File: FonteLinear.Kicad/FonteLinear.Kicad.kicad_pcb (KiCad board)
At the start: 2 copper layers, 26 parts, among them J1 Conn_01x03_Male, J2 Conn_01x02_Male, J3 Conn_01x02_Male, J4 Conn_01x02_Male, J5 Conn_01x02_Male, U1 LM317_TO39, U2 LM7805_TO220, U3 LM7815_TO220, U4 LM7915_TO220

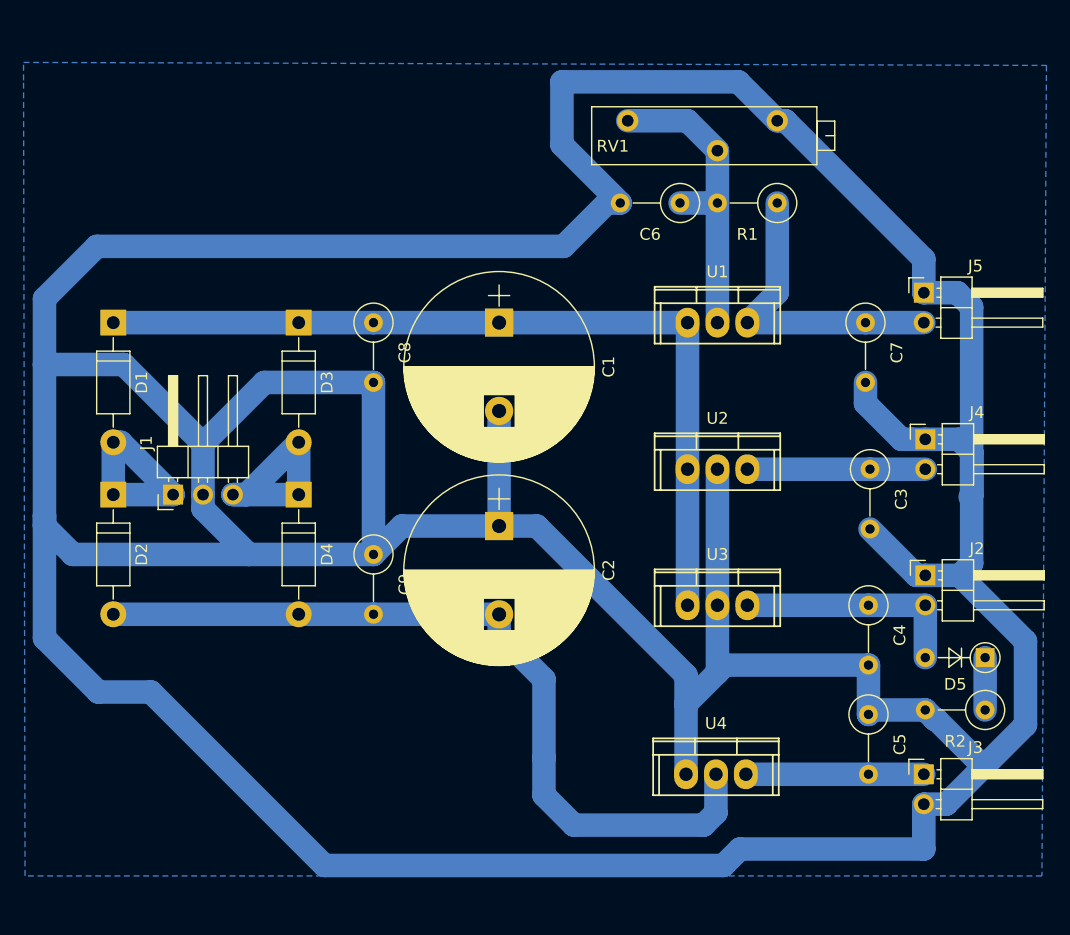
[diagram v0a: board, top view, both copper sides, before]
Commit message: Add files via upload
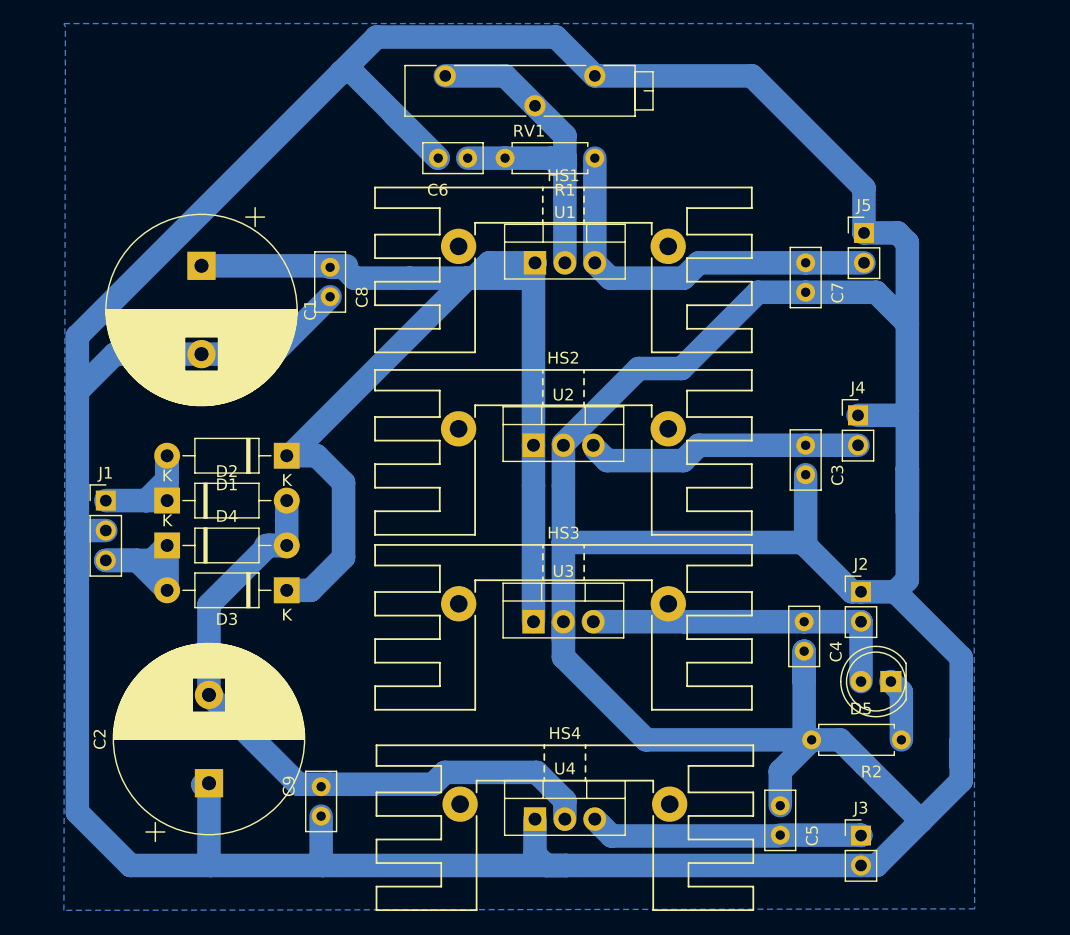
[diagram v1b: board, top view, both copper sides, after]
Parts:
- added HS1: Heatsink, Heatsinks:Heatsink_Stonecold_HS-132_32x14mm_2xFixation1.5mm, F.Cu at (236.6, 106.7)
- added HS2: Heatsink, Heatsinks:Heatsink_Stonecold_HS-132_32x14mm_2xFixation1.5mm, F.Cu at (236.6, 122.2)
- added HS3: Heatsink, Heatsinks:Heatsink_Stonecold_HS-132_32x14mm_2xFixation1.5mm, F.Cu at (236.6, 137.0)
- added HS4: Heatsink, Heatsinks:Heatsink_Stonecold_HS-132_32x14mm_2xFixation1.5mm, F.Cu at (236.7, 154.1)
- C1, C2: footprint Capacitors_THT:CP_Radial_D16.0mm_P7.50mm -> Capacitor_THT:CP_Radial_D16.0mm_P7.50mm
- C3, C4, C5, C6, C7, C8, C9: footprint Resistors_THT:R_Axial_DIN0309_L9.0mm_D3.2mm_P5.08mm_Vertical -> Capacitors_THT:C_Disc_D5.0mm_W2.5mm_P2.50mm
- D1, D2, D3, D4: footprint Diodes_THT:D_DO-41_SOD81_P10.16mm_Horizontal -> Diode_THT:D_DO-41_SOD81_P10.16mm_Horizontal
- D5: footprint Diodes_THT:D_DO-35_SOD27_P5.08mm_Vertical_AnodeUp -> LEDs:LED_D5.0mm
- J1: footprint Pin_Headers:Pin_Header_Angled_1x03_Pitch2.54mm -> Connector_PinHeader_2.54mm:PinHeader_1x03_P2.54mm_Vertical
- J2, J3, J4, J5: footprint Pin_Headers:Pin_Header_Angled_1x02_Pitch2.54mm -> Connector_PinHeader_2.54mm:PinHeader_1x02_P2.54mm_Vertical
- R1, R2: footprint Resistors_THT:R_Axial_DIN0309_L9.0mm_D3.2mm_P5.08mm_Vertical -> Resistors_THT:R_Axial_DIN0207_L6.3mm_D2.5mm_P7.62mm_Horizontal
- RV1: footprint Potentiometers:Potentiometer_Trimmer_Vishay_43 -> Potentiometer_THT:Potentiometer_Bourns_3005_Horizontal
- U1, U2, U3, U4: footprint Power_Integrations:TO-220 -> Package_TO_SOT_THT:TO-220-3_Vertical
- moved C2 32.9 mm to (206.5, 152.3), turned to 90 degrees
- moved C1 25.7 mm to (205.9, 108.3)
- moved D3 22.8 mm to (213.1, 135.9), turned to 180 degrees
- moved C9 22.7 mm to (216.0, 155.1), turned to 90 degrees
- moved D1 18.6 mm to (213.1, 124.5), turned to 180 degrees
- moved C6 18.4 mm to (228.5, 99.2)
- moved U1 16.3 mm to (234.2, 108.1)
- moved R1 16.0 mm to (239.3, 99.2)
- moved RV1 16.0 mm to (226.6, 92.2)
- moved U4 15.8 mm to (234.2, 155.3)
- moved U2 15.8 mm to (234.1, 123.6)
- moved U3 15.7 mm to (234.1, 138.6)
- moved D4 12.0 mm to (202.9, 132.1), turned to 0 degrees
- moved C5 10.8 mm to (255.0, 154.2)
- moved D5 8.26 mm to (264.4, 143.6)
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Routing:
- net /Vbus+: track 72.8 -> 106.1 mm
- net GND: track 489.7 -> 475.2 mm
- net /Vbus-: track 69.1 -> 58.8 mm
- net /Vcc+15V: track 19.6 -> 27.8 mm
- net /Vcc+5V: track 15.1 -> 23.3 mm
- net /Vcc-15V: track 15.1 -> 23.1 mm
- net /VccAjustavel: track 26.2 -> 32.8 mm
- net Net-(C6-Pad1): track 26.5 -> 33.1 mm
- net Net-(D1-Pad2): track 16.4 -> 13.6 mm
- net Net-(D3-Pad2): track 17.5 -> 15.8 mm
- net Net-(D5-Pad1): track 4.45 -> 5.32 mm
